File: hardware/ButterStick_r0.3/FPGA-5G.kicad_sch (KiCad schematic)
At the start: 1 part, among them U2 ECP5UM5G_85_CABGA381

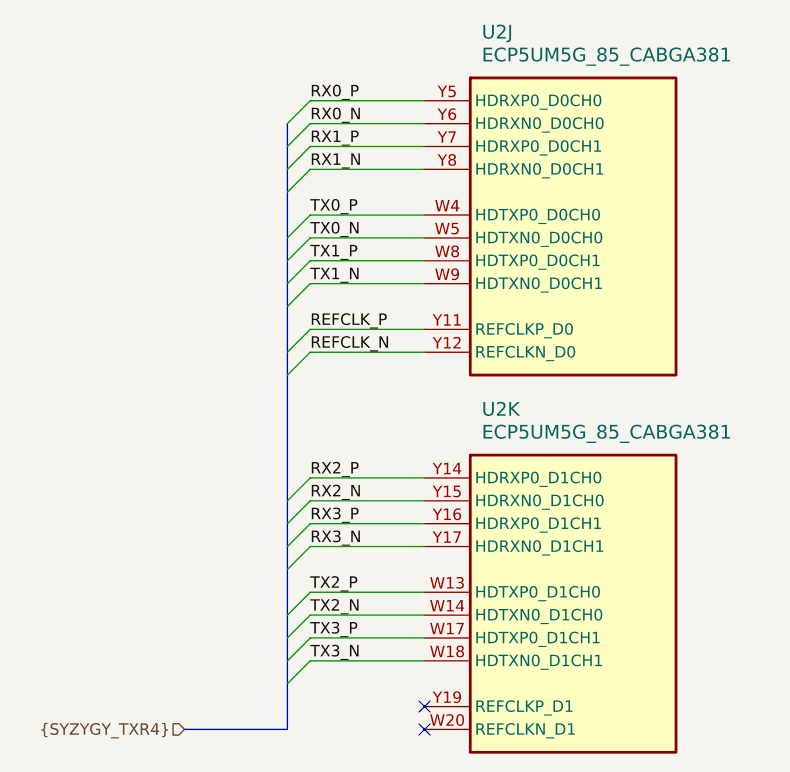
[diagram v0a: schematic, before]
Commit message: hw.r0_3: major blocks roughly routed
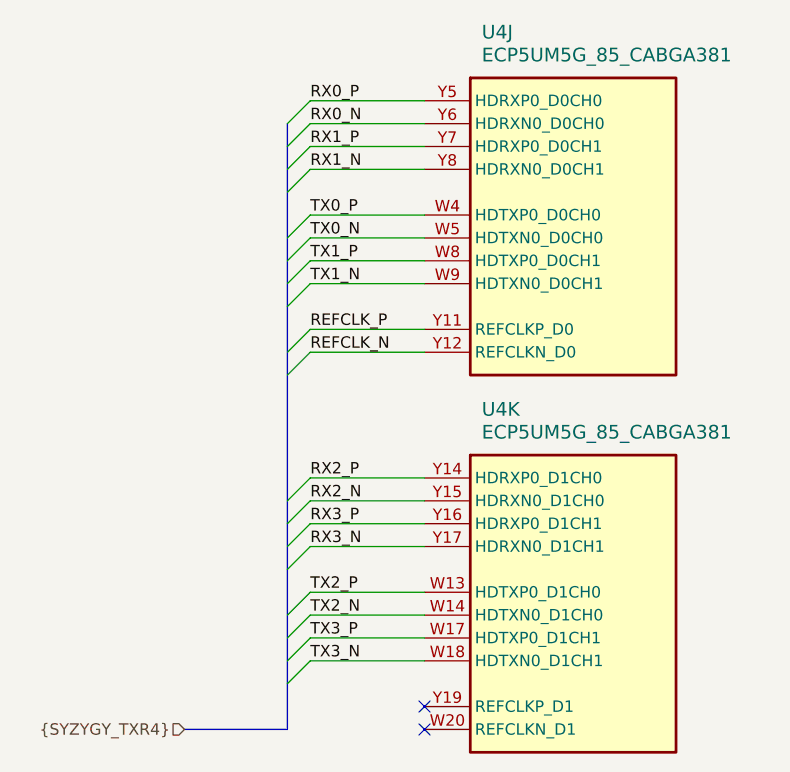
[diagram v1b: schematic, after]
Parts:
- renumbered U2 to U4
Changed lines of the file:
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@@
 (kicad_sch (version 20200512) (host eeschema "5.99.0-unknown-711fc99~101~ubuntu18.04.1")
-  (page 11 19)
+  (page 1 19)
   (paper "A4")
   (no_connect (at 77.47 137.16))
@@
   (bus (pts (xy 62.23 72.39) (xy 62.23 74.93)))
   (bus (pts (xy 62.23 74.93) (xy 62.23 80.01)))
-  (bus (pts (xy 62.23 80.01) (xy 62.23 85.09)))
-  (bus (pts (xy 62.23 85.09) (xy 62.23 90.17)))
-  (bus (pts (xy 62.23 90.17) (xy 62.23 97.79)))
-  (bus (pts (xy 62.23 97.79) (xy 62.23 114.3)))
-  (bus (pts (xy 62.23 114.3) (xy 62.23 119.38)))
-  (bus (pts (xy 62.23 119.38) (xy 62.23 127)))
-  (bus (pts (xy 62.23 127) (xy 62.23 132.08)))
-  (bus (pts (xy 62.23 132.08) (xy 62.23 139.7)))
+  (bus (pts (xy 62.23 80.01) (xy 62.23 87.63)))
+  (bus (pts (xy 62.23 87.63) (xy 62.23 92.71)))
+  (bus (pts (xy 62.23 92.71) (xy 62.23 100.33)))
+  (bus (pts (xy 62.23 100.33) (xy 62.23 116.84)))
+  (bus (pts (xy 62.23 116.84) (xy 62.23 121.92)))
+  (bus (pts (xy 62.23 121.92) (xy 62.23 129.54)))
+  (bus (pts (xy 62.23 129.54) (xy 62.23 134.62)))
+  (bus (pts (xy 62.23 134.62) (xy 62.23 139.7)))
   (label "RX0_P" (at 64.77 69.85 0)
     (effects (font (size 1.27 1.27)) (justify left bottom))
@@
   )
   (symbol (lib_id "gkl_lattice:ECP5UM5G_85_CABGA381") (at 77.47 72.39 0) (unit 10)
-    (property "Reference" "U2" (id 0) (at 83.82 62.23 0)
+    (property "Reference" "U4" (id 0) (at 83.82 62.23 0)
       (effects (font (size 1.524 1.524)) (justify left))
     )
@@
   )
   (symbol (lib_id "gkl_lattice:ECP5UM5G_85_CABGA381") (at 77.47 114.3 0) (unit 11)
-    (property "Reference" "U2" (id 0) (at 83.82 104.14 0)
+    (property "Reference" "U4" (id 0) (at 83.82 104.14 0)
       (effects (font (size 1.524 1.524)) (justify left))
     )
